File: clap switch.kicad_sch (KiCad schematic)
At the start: 14 parts, among them Q1 BC547, Q2 BC547, U1 NE555D

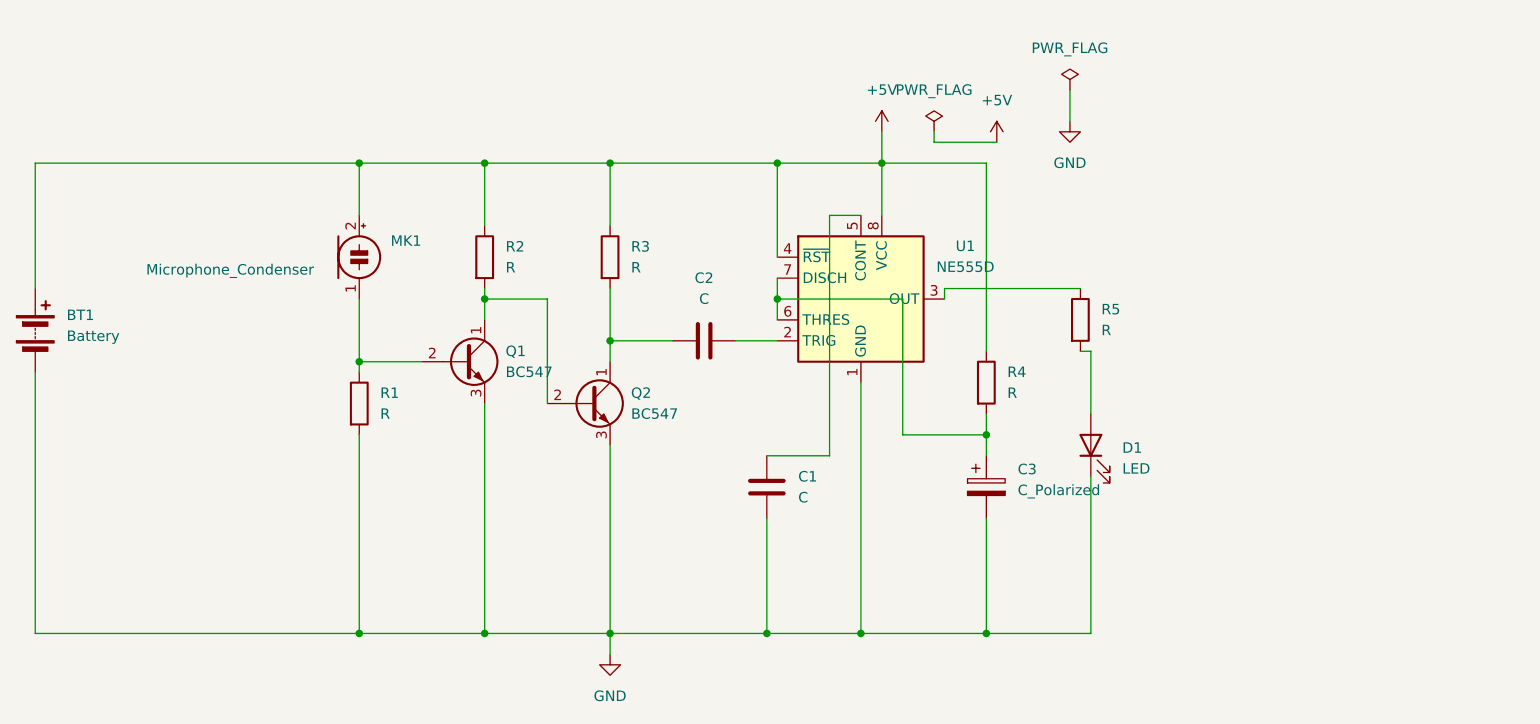
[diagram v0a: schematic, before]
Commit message: updated clap switch project
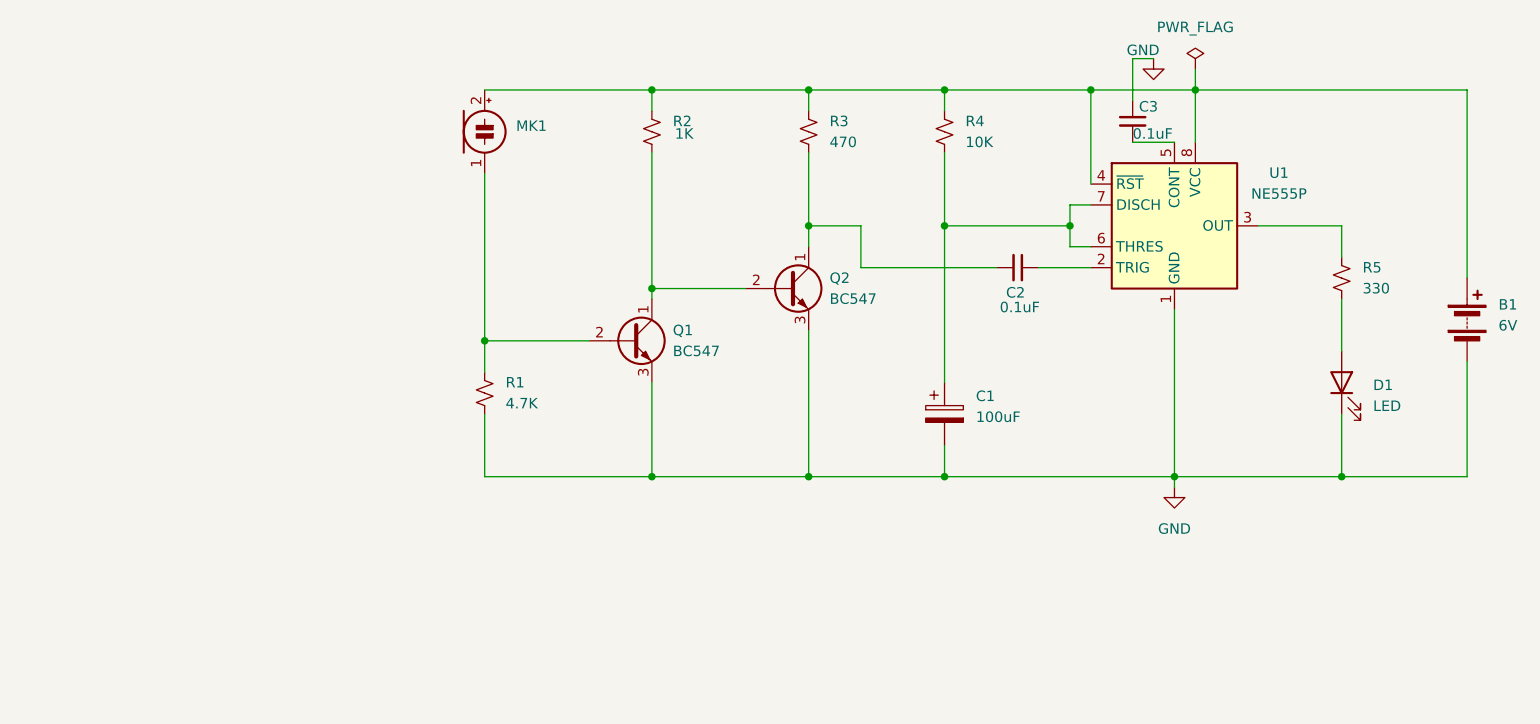
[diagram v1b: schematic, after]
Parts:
- removed BT1: Battery, Battery:BatteryHolder_Keystone_106_1x20mm, symbol Device:Battery
- removed C1, C2: C, Capacitor_THT:C_Disc_D3.4mm_W2.1mm_P2.50mm, symbol Device:C
- removed C3: C_Polarized, Capacitor_THT:CP_Radial_D4.0mm_P2.00mm, symbol Device:C_Polarized
- removed R1, R2, R3, R4, R5: R, Resistor_THT:R_Axial_DIN0207_L6.3mm_D2.5mm_P7.62mm_Horizontal, symbol Device:R
- removed U1: NE555D, Package_DIP:DIP-8_W7.62mm, symbol Timer:NE555D
- added B1: 6V, Connector_PinHeader_2.54mm:PinHeader_1x02_P2.54mm_Vertical, symbol Device:Battery
- added C1: 100uF, Capacitor_THT:CP_Axial_L10.0mm_D4.5mm_P15.00mm_Horizontal, symbol Device:C_Polarized
- added C2, C3: 0.1uF, Capacitor_THT:C_Disc_D5.0mm_W2.5mm_P2.50mm, symbol Device:C_Small
- added R1: 4.7K, Resistor_THT:R_Axial_DIN0207_L6.3mm_D2.5mm_P7.62mm_Horizontal, symbol Device:R_Small_US
- added R2: 1K, Resistor_THT:R_Axial_DIN0207_L6.3mm_D2.5mm_P7.62mm_Horizontal, symbol Device:R_Small_US
- added R3: 470, Resistor_THT:R_Axial_DIN0207_L6.3mm_D2.5mm_P7.62mm_Horizontal, symbol Device:R_Small_US
- added R4: 10K, Resistor_THT:R_Axial_DIN0207_L6.3mm_D2.5mm_P7.62mm_Horizontal, symbol Device:R_Small_US
- added R5: 330, Resistor_THT:R_Axial_DIN0207_L6.3mm_D2.5mm_P7.62mm_Horizontal, symbol Device:R_Small_US
- added U1: NE555P, Package_DIP:DIP-8_W7.62mm, symbol Timer:NE555P
- D1: footprint LED_THT:LED_D3.0mm -> LED_THT:LED_D5.0mm
- MK1: value Microphone_Condenser -> (none); footprint Connector_PinSocket_2.54mm:PinSocket_1x02_P2.54mm_Horizontal -> Connector_PinHeader_2.54mm:PinHeader_1x02_P2.54mm_Vertical
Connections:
- net GND: now also B1.2 (-), C1.2, C3.1, R1.2, U1.1 (GND)
- net at Q2.1 (C): now also C2.1, R3.2
- net at Q1.1 (C), Q2.2 (B): now also R2.2
- net at MK1.1 (-), Q1.2 (B): now also R1.1
- net at D1.2 (A): now also R5.2
- net +5V: no longer names the net of MK1.2 (+)
- net +5V: now also B1.1 (+), R2.1, R3.1, R4.1, U1.4 (~{RST}), U1.8 (VCC)
- new net: C3.2, U1.5 (CONT)
- new net: C2.2, U1.2 (TRIG)
- new net: C1.1, R4.2, U1.6 (THRES), U1.7 (DISCH)
- new net: R5.1, U1.3 (OUT)
